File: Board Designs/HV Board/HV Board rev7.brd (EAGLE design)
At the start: 118.6 x 71.4 mm, 58 parts, among them IC1 OKI-78SR, IC2 NE5532SOIC

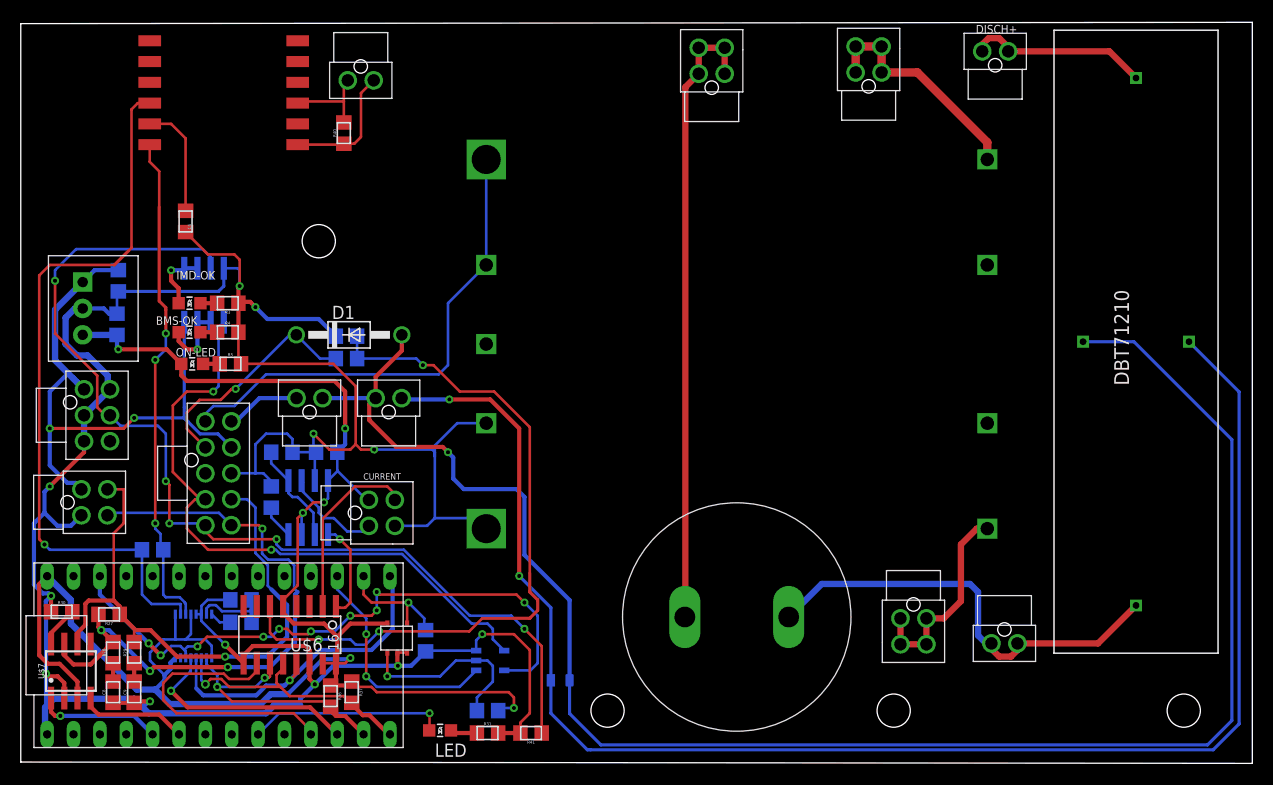
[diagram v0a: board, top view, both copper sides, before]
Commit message: Moved 6820 next to transformer
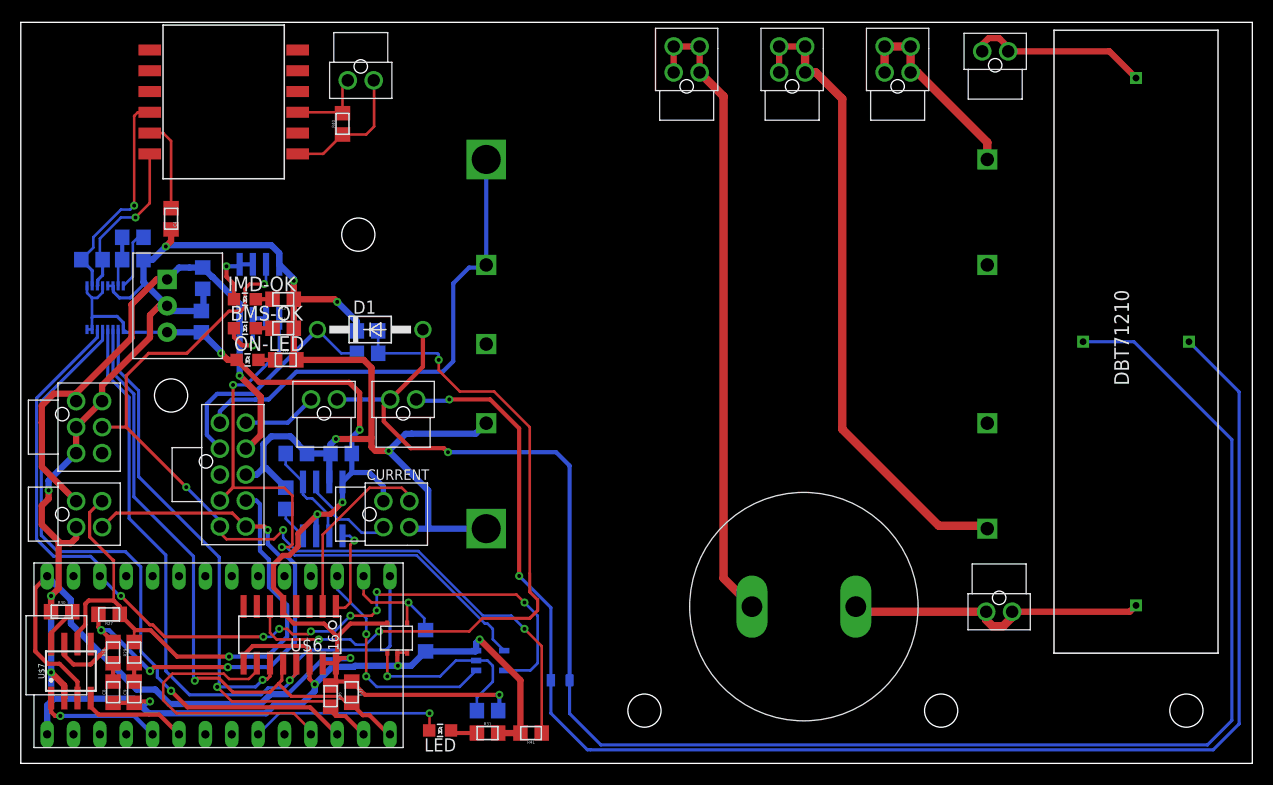
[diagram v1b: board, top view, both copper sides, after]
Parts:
- IMD: value IMD -> CONNECTOR-6NANO-FIT_VERTICAL-6
- moved HV-FUSED_1A-IMD- 53.9 mm to (94.9, 61.2), turned to 0 degrees
- moved R33 38.5 mm to (31.4, 45.3), turned to 0 degrees
- moved R34 34.4 mm to (31.4, 43.2), turned to 180 degrees
- moved U$8 32.7 mm to (30.4, 37.0)
- moved R35 28.5 mm to (27.4, 43.2)
- moved C2 8.13 mm to (38.1, 41.4)
- moved C3 8.13 mm to (38.0, 37.2)
- moved IC1 8.13 mm to (34.7, 38.7)
- moved C1 6.54 mm to (96.0, 9.76)
- moved BMS-OK 5.35 mm to (42.2, 36.6)
- moved IC2 5.35 mm to (43.6, 40.1)
- moved IMD-OK 5.35 mm to (42.2, 39.4)
- moved R3 5.35 mm to (45.8, 39.4)
- moved R4 5.35 mm to (45.8, 36.6)
- moved ON-LED 5.35 mm to (42.4, 33.5)
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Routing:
- net N$33: track 70.4 -> 21.1 mm
- net CS_LTC6820: track 21.7 -> 64.0 mm
- net HV-FUSED_1A: track 20.6 -> 61.9 mm
- net SCK: track 31.9 -> 69.1 mm
- net MISO: track 25.7 -> 61.2 mm
- net MOSI: track 26.8 -> 61.5 mm
- net N$34: track 48.3 -> 15.8 mm, vias 3 -> 1
- net +3V3: track 60.5 -> 87.7 mm, vias 10 -> 8
- net GND: track 271.2 -> 249.5 mm
- net HV+UNFUSED: track 42.9 -> 29.4 mm
- net +5V: track 171.9 -> 159.3 mm
- net OKHS: track 98.3 -> 86.2 mm, vias 5 -> 4
- net +12V: track 59.0 -> 54.7 mm, vias 2 -> 1
- net N$31: track 2.12 -> 5.79 mm
- net BMS_OK: track 62.3 -> 59.1 mm
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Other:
- outline, holes or cut-outs redrawn
- board text added: "IMD"
